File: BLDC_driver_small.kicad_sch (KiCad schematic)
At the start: 58 parts, among them J1 1x02 Terminal, J2 1x03 Terminal, Q1 Q_PMOS_GDS, SW1 RST_SW, SW2 SW_SPDT, U1 NCP786L, U2 L6230Q, U3 ADS131M03IPWR, U4 STM32F030K6Tx, Y1 16MHz

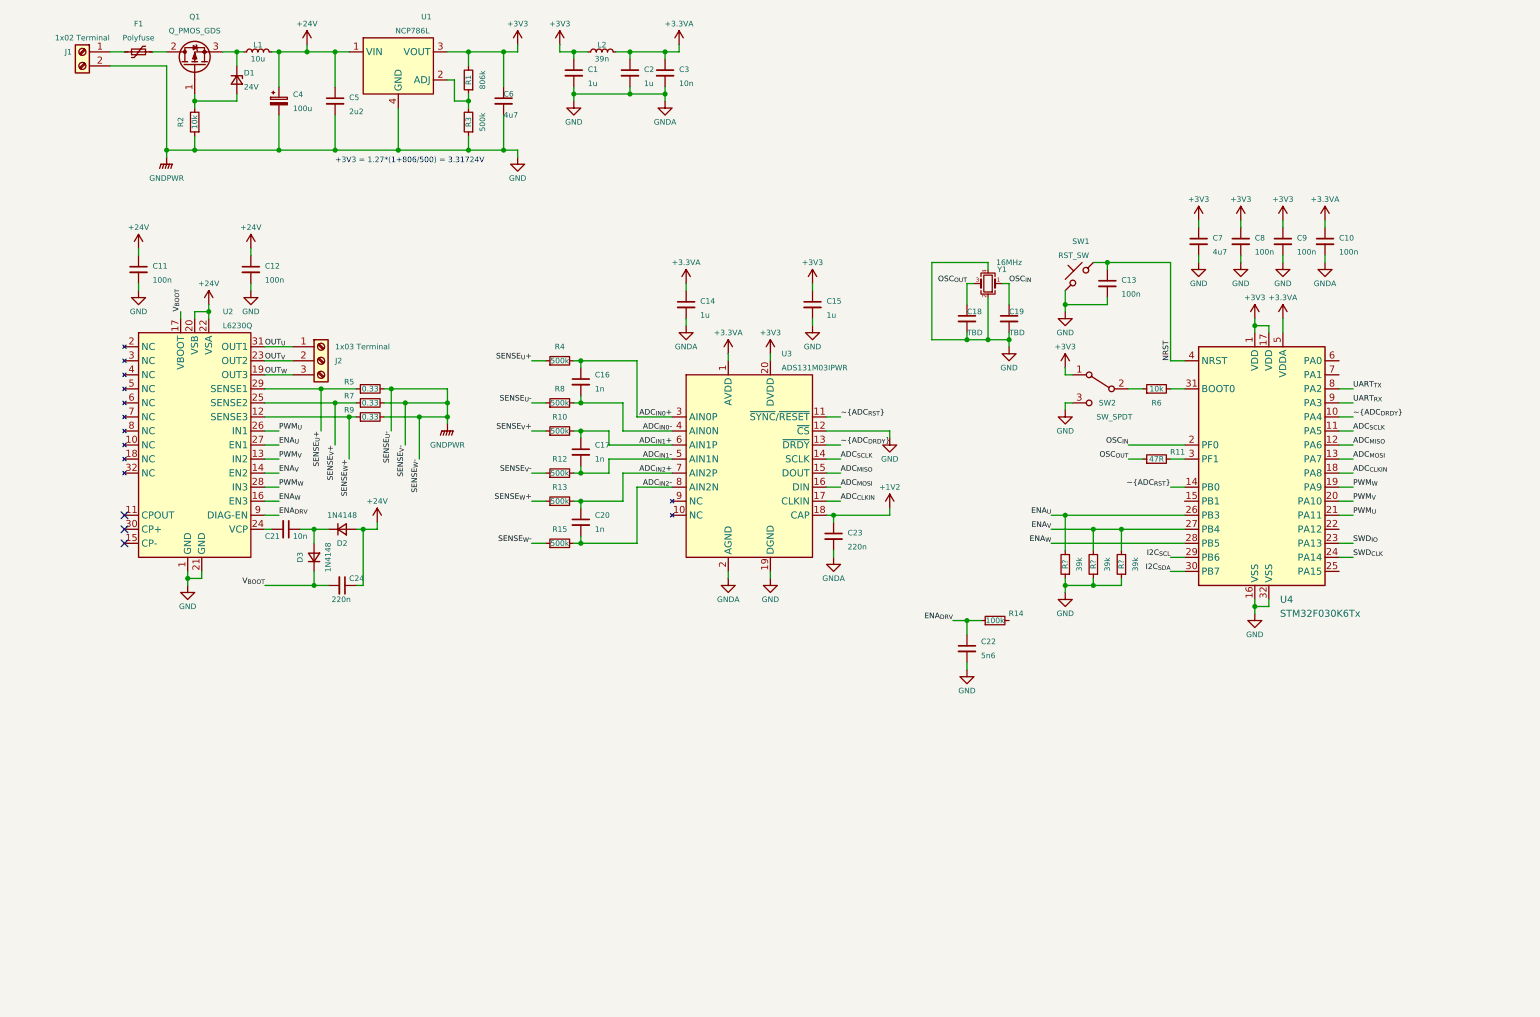
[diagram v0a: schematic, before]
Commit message: 130323-3 fullchange
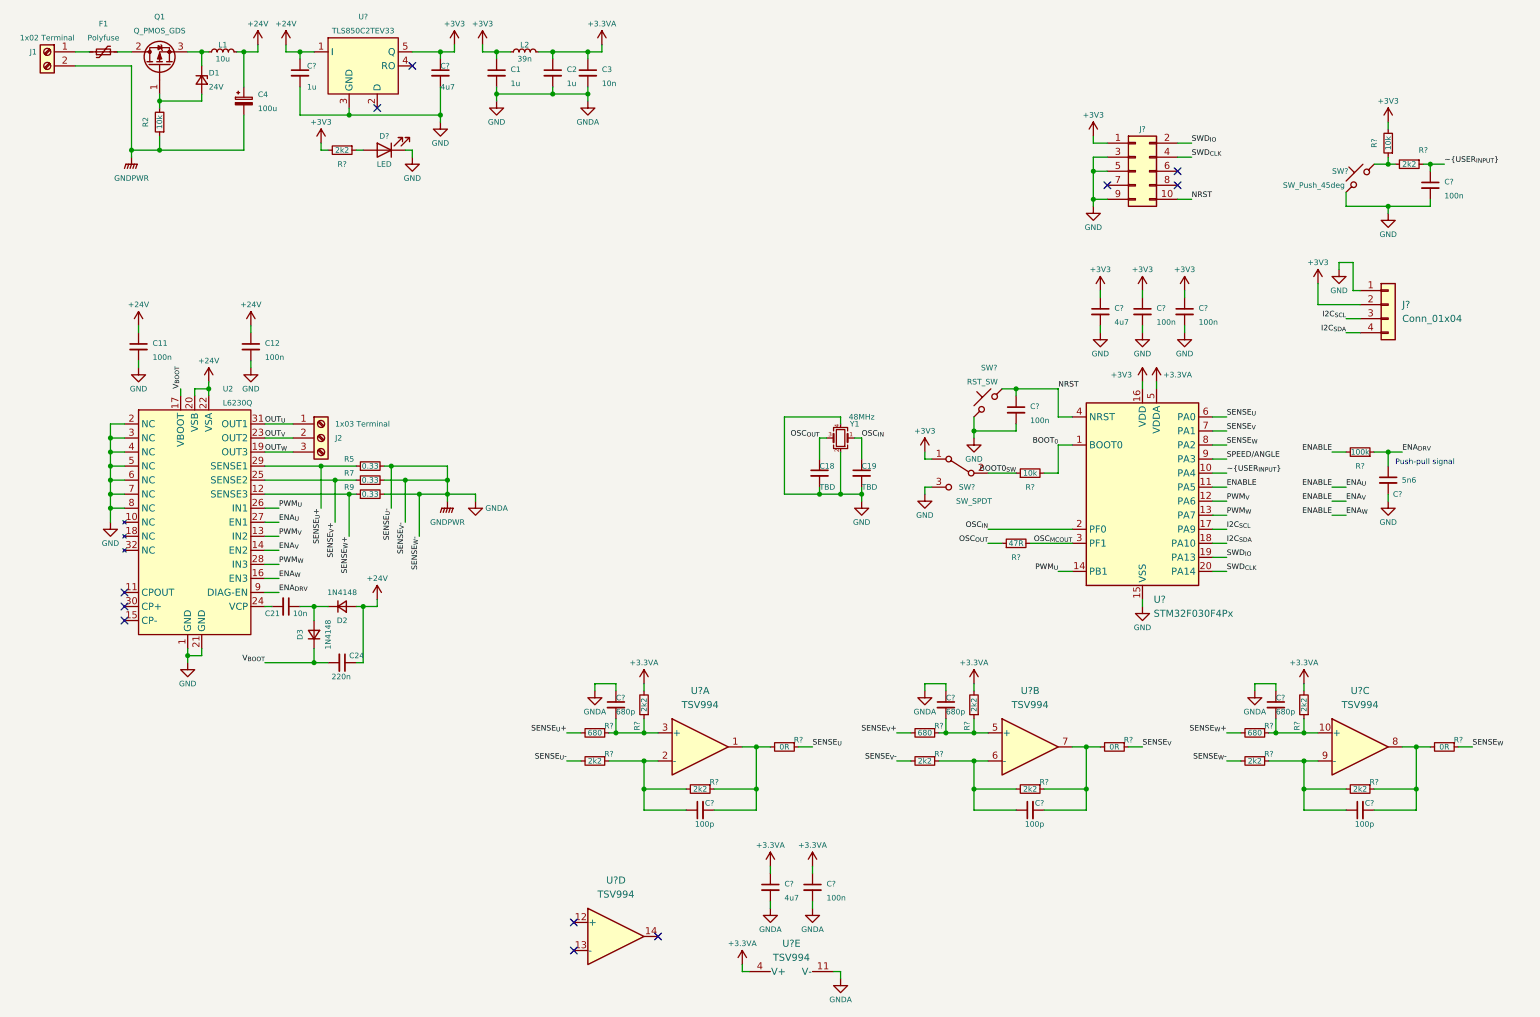
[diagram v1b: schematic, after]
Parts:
- removed C10, C13, C8, C9: 100n, Capacitor_SMD:C_0402_1005Metric, symbol Device:C_Small
- removed C14, C15: 1u, Capacitor_SMD:C_0402_1005Metric, symbol Device:C_Small
- removed C16, C17, C20: 1n, Capacitor_SMD:C_0402_1005Metric, symbol Device:C_Small
- removed C22: 5n6, Capacitor_SMD:C_0402_1005Metric, symbol Device:C_Small
- removed C23: 220n, Resistor_SMD:R_0402_1005Metric, symbol Device:C_Small
- removed C5: 2u2, Capacitor_SMD:C_0805_2012Metric, symbol Device:C_Small
- removed C6, C7: 4u7, Capacitor_SMD:C_0603_1608Metric, symbol Device:C_Small
- removed R1: 806k, Resistor_SMD:R_0603_1608Metric, symbol Device:R_Small
- removed R10, R12, R13, R15, R4, R8: 500k, Resistor_SMD:R_0402_1005Metric, symbol Device:R_Small
- removed R11: 47R, Resistor_SMD:R_0402_1005Metric, symbol Device:R_Small
- removed R14: 100k, Resistor_SMD:R_0603_1608Metric, symbol Device:R_Small
- removed R3: 500k, Resistor_SMD:R_0603_1608Metric, symbol Device:R_Small
- removed R6: 10k, Resistor_SMD:R_0603_1608Metric, symbol Device:R_Small
- removed R? (x3): 39k, Resistor_SMD:R_0603_1608Metric, symbol Device:R_Small
- removed SW1: RST_SW, Button_Switch_SMD:SW_SPST_B3S-1000, symbol Switch:SW_Push_45deg
- removed SW2: SW_SPDT, Button_Switch_SMD:SW_SPDT_PCM12, symbol Switch:SW_SPDT
- removed U1: NCP786L, Package_TO_SOT_SMD:SOT-223, symbol fraciscoestar:NCP786L
- removed U3: ADS131M03IPWR, Package_SO:TSSOP-20_4.4x6.5mm_P0.65mm, symbol fraciscoestar:ADS131M03IPWR
- removed U4: STM32F030K6Tx, Package_QFP:LQFP-32_7x7mm_P0.8mm, symbol MCU_ST_STM32F0:STM32F030K6Tx
- added C? (x5): 100n, Capacitor_SMD:C_0402_1005Metric, symbol Device:C_Small
- added C? (x3): 680p, Capacitor_SMD:C_0402_1005Metric, symbol Device:C_Small
- added C? (x3): 100p, Capacitor_SMD:C_0402_1005Metric, symbol Device:C_Small
- added C? (x3): 4u7, Capacitor_SMD:C_0603_1608Metric, symbol Device:C_Small
- added C?: 5n6, Capacitor_SMD:C_0402_1005Metric, symbol Device:C_Small
- added C?: 1u, Capacitor_SMD:C_0805_2012Metric, symbol Device:C_Small
- added D?: LED, symbol Device:LED
- added J?: Conn_01x04, symbol Connector_Generic:Conn_01x04
- added J?: Conn_02x05_Odd_Even, symbol Connector_Generic:Conn_02x05_Odd_Even
- added R? (x10): 2k2, Resistor_SMD:R_1210_3225Metric, symbol Device:R_Small
- added R? (x3): 680, Resistor_SMD:R_1210_3225Metric, symbol Device:R_Small
- added R? (x2): 10k, Resistor_SMD:R_0603_1608Metric, symbol Device:R_Small
- added R? (x3): 0R, Resistor_SMD:R_1210_3225Metric, symbol Device:R_Small
- added R?: 2k2, Resistor_SMD:R_0603_1608Metric, symbol Device:R_Small
- added R?: 47R, Resistor_SMD:R_0402_1005Metric, symbol Device:R_Small
- added R?: 100k, Resistor_SMD:R_0603_1608Metric, symbol Device:R_Small
- added SW?: SW_SPDT, Button_Switch_SMD:SW_SPDT_PCM12, symbol Switch:SW_SPDT
- added SW?: SW_Push_45deg, symbol Switch:SW_Push_45deg
- added SW?: RST_SW, Button_Switch_SMD:SW_SPST_B3S-1000, symbol Switch:SW_Push_45deg
- added U?: TLS850C2TEV33, Package_TO_SOT_SMD:TO-252-5_TabPin3, symbol fraciscoestar:TLS850C2TEV33
- added U? (x5): TSV994, symbol Amplifier_Operational:TSV994
- added U?: STM32F030F4Px, Package_SO:TSSOP-20_4.4x6.5mm_P0.65mm, symbol MCU_ST_STM32F0:STM32F030F4Px
- Y1: value 16MHz -> 48MHz
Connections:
- net ENA_{V} is gone; now on net ENABLE: U2.14 (EN2)
- net ENA_{W} is gone; now on net ENABLE: U2.16 (EN3)
- net +24V: now also C?.1, U?.1 (I)
- net +3.3VA: now also C?.1, C?.1, R?.2, R?.2, R?.2, U?.4 (V+), U?.5 (VDDA)
- net +3V3: now also C?.1, C?.1, C?.1, C?.1, J?.1 (Pin_1), J?.2 (Pin_2), R?.2, R?.2, SW?.1 (A), U?.16 (VDD), U?.5 (Q)
- net ENA_{DRV}: now also C?.1, R?.1
- net GND: now also U2.2 (NC), U2.3 (NC), U2.4 (NC), U2.5 (NC), U2.6 (NC), U2.7 (NC), U2.8 (NC), C?.1, C?.1, C?.1, C?.2, C?.2, C?.2, C?.2, C?.2, C?.2, C?.2, C?.2, C?.2, C?.2, D?.1 (K), J?.1 (Pin_1), J?.3 (Pin_3), J?.5 (Pin_5), J?.9 (Pin_9), R?.2, R?.2, R?.2, SW?.1, SW?.1, SW?.3 (C), U?.11 (V-), U?.15 (VSS), U?.3 (GND)
- net I2C_{SCL}: now also J?.3 (Pin_3), U?.17 (PA9)
- net I2C_{SDA}: now also J?.4 (Pin_4), U?.18 (PA10)
- net NRST: now also C?.1, J?.10 (Pin_10), SW?.2, U?.4 (NRST)
- net OSC_{IN}: now also U?.2 (PF0)
- net OSC_{OUT}: now also R?.1
- net PWM_{U}: now also U?.14 (PB1)
- net PWM_{V}: now also U?.12 (PA6)
- net PWM_{W}: now also U?.13 (PA7)
- net SENSE_{U}+: now also R?.2
- net SENSE_{V}+: now also R?.2
- net SENSE_{W}+: now also R?.2
- net SWD_{CLK}: now also J?.4 (Pin_4), U?.20 (PA14)
- net SWD_{IO}: now also J?.2 (Pin_2), U?.19 (PA13)
- net ENA_{U} renamed ENABLE
- net ENABLE: now also R?.2, U?.11 (PA5)
- new net: C?.2, R?.1, R?.2, U?.7
- new net: C?.1, R?.1, R?.2, U?.6 (-)
- new net: C?.2, R?.1, R?.1, U?.3 (+)
- new net: C?.2, R?.1, R?.2, U?.1
- new net: C?.1, R?.1, R?.2, U?.2 (-)
- new net: C?.2, R?.1, R?.1, U?.5 (+)
- new net: C?.2, R?.1, R?.1, U?.10 (+)
- new net: C?.2, R?.1, R?.2, U?.8
- new net: C?.1, R?.1, R?.2, U?.9 (-)
- new net: R?.1, R?.2, SW?.2
- new net: D?.2 (A), R?.1
- new net BOOT0_{SW}: R?.1, SW?.2 (B)
- new net BOOT_{0}: R?.2, U?.1 (BOOT0)
- new net OSC_{MCOUT}: R?.2, U?.3 (PF1)
- new net SENSE_{U}: R?.1, U?.6 (PA0)
- new net SENSE_{V}: R?.1, U?.7 (PA1)
- new net SENSE_{W}: R?.1, U?.8 (PA2)
- new net SPEED/ANGLE: U?.9 (PA3)
- new net ~{USER_{INPUT}}: C?.1, R?.1, U?.10 (PA4)
- no-connect marks 3 -> 11
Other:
- note added: "Push-pull signal"
- note removed: "+3V3 = 1.27*(1+806/500) = 3.31724V"
- moved on the sheet: C1, C11, C12, C18, C19, C2, C21, C24, C3, C4, D1, D2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
